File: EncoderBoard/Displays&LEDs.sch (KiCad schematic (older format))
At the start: 33 parts, among them U10 Display_OLED_128x32_I2C, U11 Display_OLED_128x32_I2C, U12 Display_OLED_128x32_I2C, U13 Display_OLED_128x32_I2C, U14 Display_OLED_128x32_I2C, U15 Display_OLED_128x32_I2C, U16 Display_OLED_128x32_I2C, U17 Display_OLED_128x32_I2C, U9 Display_OLED_128x32_I2C

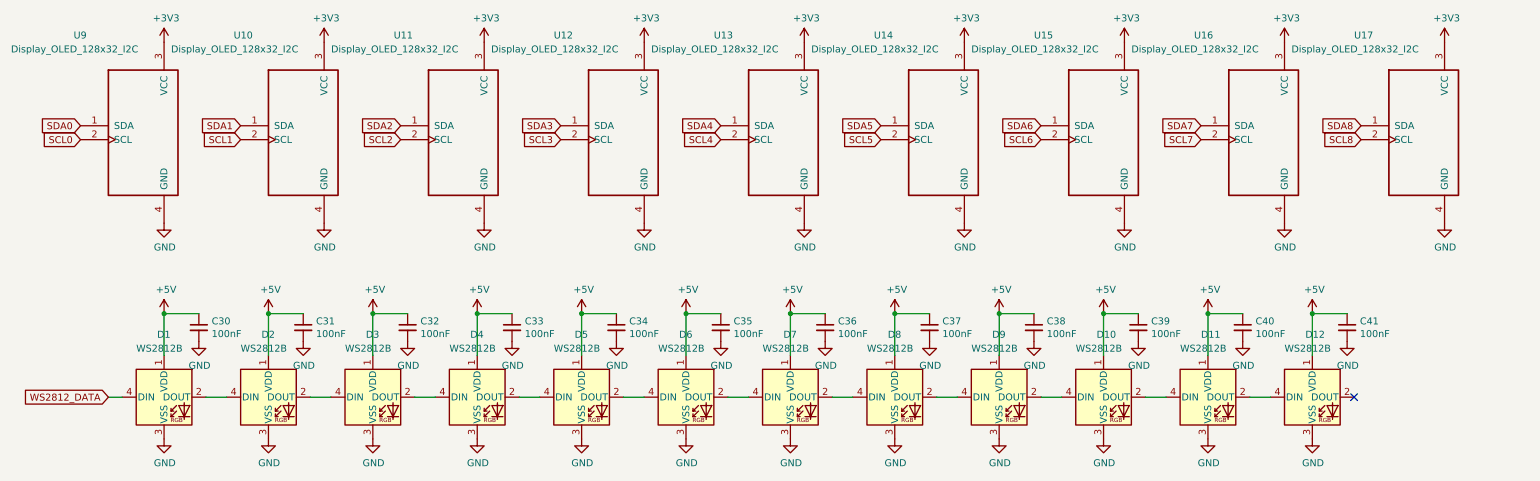
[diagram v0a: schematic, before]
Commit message: Final version of Rev A board.
- Fixed up address pins on some chips.
- Added some additional bypass capacitors.
- Fixed up some broken footprint references.
- Some minor layout adjustments.
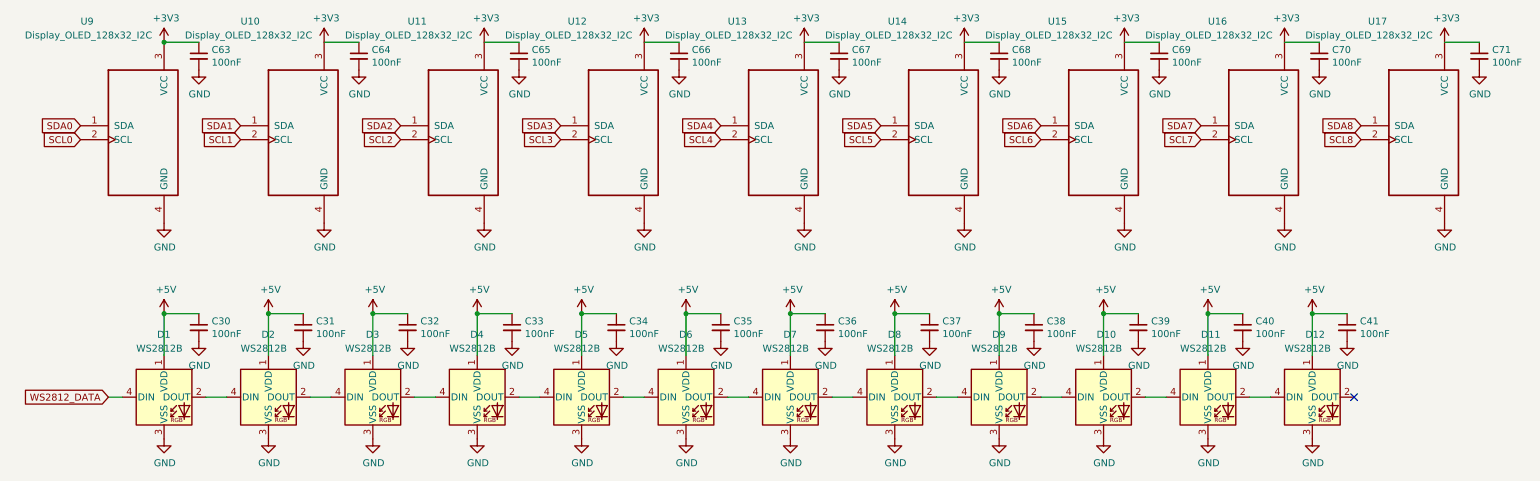
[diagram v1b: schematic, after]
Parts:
- added C63, C64, C65, C66, C67, C68, C69, C70, C71: 100nF, Capacitor_BG:C_0805_2012Metric, symbol Device:C_Small
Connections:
- net +3V3: now also C63.1, C64.1, C65.1, C66.1, C67.1, C68.1, C69.1, C70.1, C71.1
- net GND: now also C63.2, C64.2, C65.2, C66.2, C67.2, C68.2, C69.2, C70.2, C71.2
